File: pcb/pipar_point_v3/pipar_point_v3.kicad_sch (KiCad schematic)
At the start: 11 parts

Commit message: adds a proper battery connector
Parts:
- U10, U9: now left out of the parts list
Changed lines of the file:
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@@
 		(unit 1)
 		(exclude_from_sim no)
-		(in_bom yes)
+		(in_bom no)
 		(on_board yes)
 		(dnp no)
@@
 		(unit 1)
 		(exclude_from_sim no)
-		(in_bom yes)
+		(in_bom no)
 		(on_board yes)
 		(dnp no)

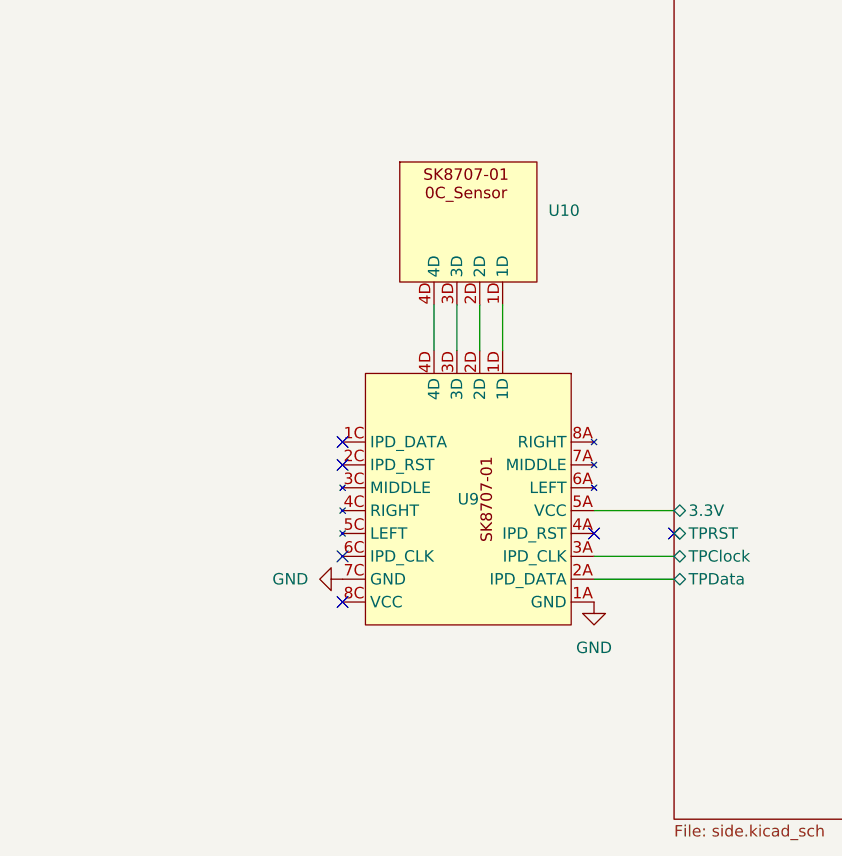
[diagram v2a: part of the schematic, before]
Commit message: Adds trackpoint reset GPIO Fix floating led 15 and 35 (mirrored)
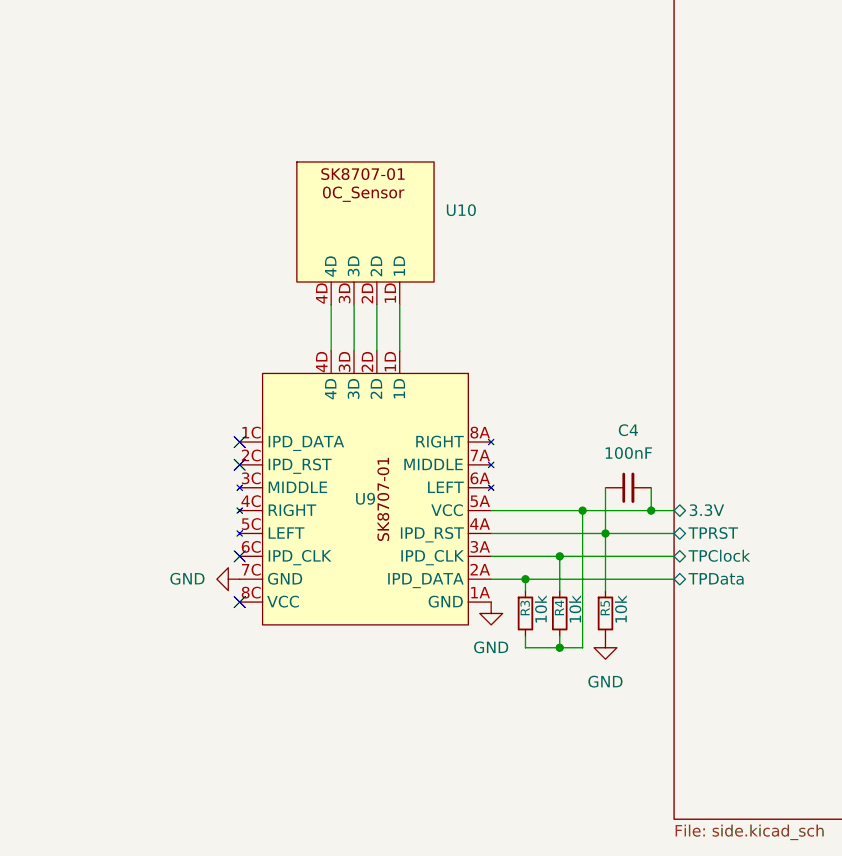
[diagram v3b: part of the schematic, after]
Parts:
- added C4: 100nF, Capacitor_SMD:C_0603_1608Metric, symbol Device:C_Small
- added R3, R4, R5: 10k, Resistor_SMD:R_0603_1608Metric, symbol Device:R_Small
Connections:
- net GND: now also R5.2
- net Side-Right/3.3V: now also C4.2, R3.2, R4.2
- net Side-Right/TPClock: now also R4.1
- net Side-Right/TPData: now also R3.1
- net Side-Right/TPRST: now also U9.4A (IPD_RST), C4.1, R5.1
- no-connect marks 10 -> 8
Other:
- moved on the sheet: U10, U9
